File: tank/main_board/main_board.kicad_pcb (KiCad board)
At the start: 2 copper layers, 66.5 x 56.2 mm, 41 parts, among them J1 PowerOut, J10 PowerMotor, J11 SigOut, J12 Spk, J13 LEDs, J14 M0, J15 M1, J16 M2, J2 PowerIn, J3 Encoder0, J4 Encoder1, J5 Encoder2, J6 Encoder3, J7 Bump0, J8 Bump1, J9 Programming Header, U1 L7805, U2 ATMEGA328P-PU, U3 SN74HC595, U4 L293D, U5 L293D, Y1 Crystal

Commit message: debug
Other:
- net class Default removed
- net class Motor removed

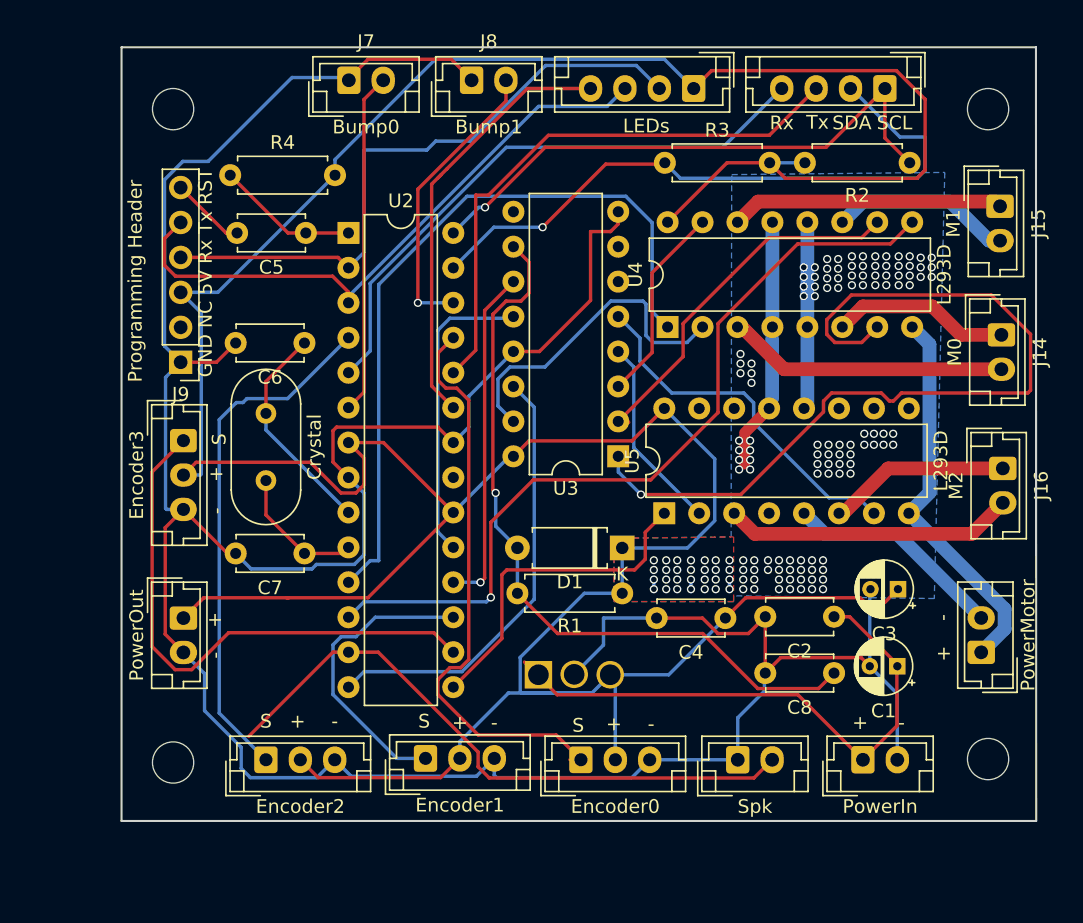
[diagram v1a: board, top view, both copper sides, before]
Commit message: Main Board v0.12
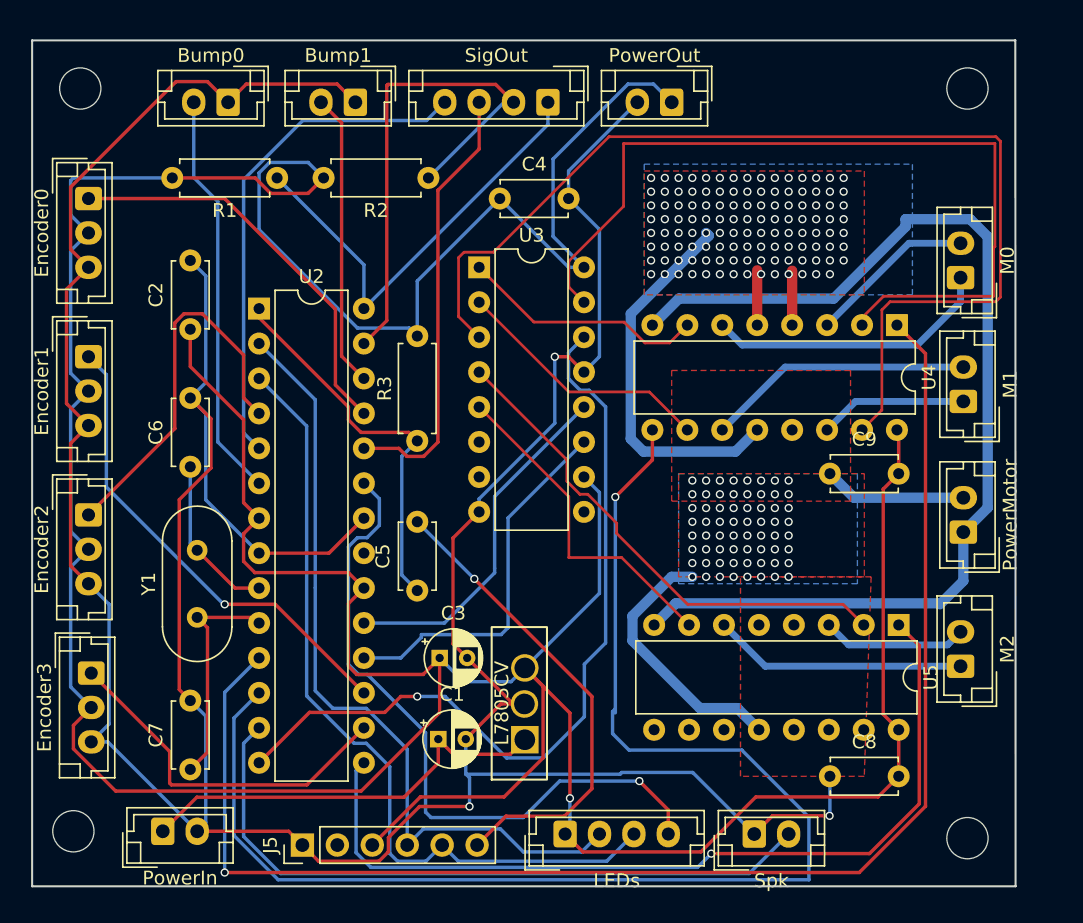
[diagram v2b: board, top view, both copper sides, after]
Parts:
- removed ?: , 
- removed D1: D, custom:D_A-405_P7.62mm_Horizontal
- removed R4: R10, custom:R_Axial_DIN0207_L6.3mm_D2.5mm_P7.62mm_Horizontal
- removed the REF** at (160.5, 125.2)
- removed the REF** at (160.5, 78.0)
- removed the REF** at (101.2, 125.5)
- removed the REF** at (101.2, 78.0)
- added C9: 100nF, custom:C_Disc_D4.7mm_W2.5mm_P5.00mm, F.Cu at (149.0, 104.5)
- added REF**: MountingHole_3mm, custom:MountingHole_3mm, F.Cu at (94.5, 76.5)
- added REF**: MountingHole_3mm, custom:MountingHole_3mm, F.Cu at (159.0, 76.5)
- added REF**: MountingHole_3mm, custom:MountingHole_3mm, F.Cu at (94.0, 130.5)
- added REF**: MountingHole_3mm, custom:MountingHole_3mm, F.Cu at (159.0, 131.0)
- C1: value CP1 -> 10uF
- C2: value C2 -> 100nF
- C3: value CP3 -> 10uF
- C4: value C4 -> 100nF
- C5, C8: value C_Small -> 100nF
- C6: value C6 -> 22pF
- C7: value C7 -> 22pF
- J1: value PowerOut -> Encoder0; footprint custom:JST_EH_B2B-EH-A_1x02_P2.50mm_Vertical -> custom:JST_EH_B3B-EH-A_1x03_P2.50mm_Vertical
- J11: value SigOut -> M0; footprint custom:JST_EH_B4B-EH-A_1x04_P2.50mm_Vertical -> custom:JST_EH_B2B-EH-A_1x02_P2.50mm_Vertical
- J12: value Spk -> M1
- J13: value LEDs -> M2; footprint custom:JST_EH_B4B-EH-A_1x04_P2.50mm_Vertical -> custom:JST_EH_B2B-EH-A_1x02_P2.50mm_Vertical
- J14: value M0 -> Spk
- J15: value M1 -> LEDs; footprint custom:JST_EH_B2B-EH-A_1x02_P2.50mm_Vertical -> custom:JST_EH_B4B-EH-A_1x04_P2.50mm_Vertical
- J16: value M2 -> SigOut; footprint custom:JST_EH_B2B-EH-A_1x02_P2.50mm_Vertical -> custom:JST_EH_B4B-EH-A_1x04_P2.50mm_Vertical
- J2: value PowerIn -> Encoder1; footprint custom:JST_EH_B2B-EH-A_1x02_P2.50mm_Vertical -> custom:JST_EH_B3B-EH-A_1x03_P2.50mm_Vertical
- J3: value Encoder0 -> Encoder2
- J4: value Encoder1 -> Encoder3
- J5: value Encoder2 -> Programming Header; footprint custom:JST_EH_B3B-EH-A_1x03_P2.50mm_Vertical -> custom:PinHeader_1x06_P2.54mm_Vertical
- J6: value Encoder3 -> Bump0; footprint custom:JST_EH_B3B-EH-A_1x03_P2.50mm_Vertical -> custom:JST_EH_B2B-EH-A_1x02_P2.50mm_Vertical
- J7: value Bump0 -> Bump1
- J8: value Bump1 -> PowerOut
- J9: value Programming Header -> PowerIn; footprint custom:PinHeader_1x06_P2.54mm_Vertical -> custom:JST_EH_B2B-EH-A_1x02_P2.50mm_Vertical
- R1: value R -> 10k
- R2: value R7 -> 10k
- R3: value R6 -> 10k
- U1: footprint Custom:L7805CV -> custom:L7805CV
- moved J2 63.5 mm to (95.1, 96.0), turned to -90 degrees
- moved J15 55.5 mm to (129.8, 130.7), turned to 0 degrees
- moved G*** 54.6 mm to (103.6, 81.3)
- moved C2 51.3 mm to (102.5, 94.0), turned to 90 degrees
- moved J13 46.3 mm to (158.5, 118.5), turned to 90 degrees
- moved J16 42.5 mm to (128.5, 77.5), turned to 180 degrees
- moved J14 40.5 mm to (143.5, 130.7), turned to 0 degrees
- moved J3 40.0 mm to (95.1, 107.5), turned to -90 degrees
- moved R1 39.3 mm to (108.8, 83.0)
- moved R2 35.0 mm to (119.8, 83.0)
- moved C4 34.6 mm to (125.0, 84.5), turned to 0 degrees
- moved J9 34.1 mm to (100.5, 130.5), turned to 0 degrees
- moved C1 33.8 mm to (120.5, 123.8), turned to 0 degrees
- moved C3 33.7 mm to (120.6, 117.9), turned to 0 degrees
- moved J1 31.3 mm to (95.1, 84.5)
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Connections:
- C2 pad 1: 9V -> 4.5V
- C8 pad 1: Net-(C8-Pad1) -> GND
- C8 pad 2: GND -> 4.5V
- J1 pad 1: 4.5V -> Encoder0
- J1 pad 2: GND -> 4.5V
- J10 pad 2: Gm -> GND
- J11 pad 1: SCL -> Net-(J11-Pad1)
- J11 pad 2: SDA -> Net-(J11-Pad2)
- J12 pad 1: GND -> Net-(J12-Pad1)
- J12 pad 2: SPK -> Net-(J12-Pad2)
- J13 pad 1: 4.5V -> Net-(J13-Pad1)
- J13 pad 2: LED0 -> Net-(J13-Pad2)
- J14 pad 1: Net-(J14-Pad1) -> GND
- J14 pad 2: Net-(J14-Pad2) -> SPK
- J15 pad 1: Net-(J15-Pad1) -> 4.5V
- J15 pad 2: Net-(J15-Pad2) -> LED0
- J16 pad 1: Net-(J16-Pad1) -> SCL
- J16 pad 2: Net-(J16-Pad2) -> SDA
- J2 pad 1: 9V -> Encoder1
- J2 pad 2: GND -> 4.5V
- J3 pad 1: Encoder0 -> Encoder2
- J4 pad 1: Encoder1 -> Encoder3
- J5 pad 1: Encoder2 -> GND
- J5 pad 2: 4.5V -> unconnected-(J5-Pad2)
- J5 pad 3: GND -> 4.5V
- J6 pad 1: Encoder3 -> GND
- J6 pad 2: 4.5V -> Bump0
- J7 pad 2: Bump0 -> Bump1
- J8 pad 1: GND -> 4.5V
- J8 pad 2: Bump1 -> GND
- J9 pad 1: GND -> 9V
- J9 pad 2: Net-(J9-Pad2) -> GND
- R1 pad 1: 4.5V -> SCL
- R1 pad 2: Net-(C8-Pad1) -> 4.5V
- R2 pad 1: SCL -> SDA
- R3 pad 1: SDA -> Net-(C5-Pad1)
- U2 pad 21: Net-(U2-Pad21) -> unconnected-(U2-Pad21)
- U3 pad 10: Net-(C8-Pad1) -> 4.5V
- U3 pad 6: Net-(U3-Pad6) -> unconnected-(U3-Pad6)
- U3 pad 7: Net-(U3-Pad7) -> unconnected-(U3-Pad7)
- U3 pad 9: Net-(U3-Pad9) -> unconnected-(U3-Pad9)
- U4 pad 11: Net-(J15-Pad2) -> Net-(J12-Pad2)
- U4 pad 12: Gm -> GND
- U4 pad 13: Gm -> GND
- U4 pad 14: Net-(J15-Pad1) -> Net-(J12-Pad1)
- U4 pad 3: Net-(J14-Pad2) -> Net-(J11-Pad2)
- U4 pad 4: Gm -> GND
- U4 pad 5: Gm -> GND
- U4 pad 6: Net-(J14-Pad1) -> Net-(J11-Pad1)
- U5 pad 10: Net-(U5-Pad10) -> unconnected-(U5-Pad10)
- U5 pad 11: Net-(U5-Pad11) -> unconnected-(U5-Pad11)
- U5 pad 12: Gm -> GND
- U5 pad 13: Gm -> GND
- U5 pad 14: Net-(U5-Pad14) -> unconnected-(U5-Pad14)
- U5 pad 15: Net-(U5-Pad15) -> unconnected-(U5-Pad15)
- U5 pad 3: Net-(J16-Pad2) -> Net-(J13-Pad2)
- U5 pad 4: Gm -> GND
- U5 pad 5: Gm -> GND
- U5 pad 6: Net-(J16-Pad1) -> Net-(J13-Pad1)
- U5 pad 9: Net-(U5-Pad9) -> unconnected-(U5-Pad9)
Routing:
- net GND: track 228.1 -> 334.4 mm, vias 0 -> 186
- net M1-: track 14.5 -> 79.2 mm
- net Net-(C8-Pad1): track 54.5 -> 0.00 mm, vias 1 -> 0
- net M0PWM: track 54.3 -> 105.4 mm, vias 0 -> 1
- net Vm: track 28.4 -> 77.9 mm
- net Gm: track 48.4 -> 0.00 mm, vias 142 -> 0
- net 4.5V: track 272.2 -> 319.9 mm, vias 0 -> 1
- net M0-: track 62.1 -> 18.0 mm, vias 1 -> 0
- net M1PWM: track 59.9 -> 99.2 mm
- net M2PWM: track 24.4 -> 63.7 mm, vias 0 -> 1
- net M0+: track 24.2 -> 62.5 mm
- net Net-(C5-Pad2): track 5.47 -> 34.7 mm, vias 0 -> 1
- net SERIAL_DATA: track 32.3 -> 58.9 mm, vias 0 -> 1
- net M2+: track 14.2 -> 36.9 mm
- net Net-(J16-Pad2): track 21.1 -> 0.00 mm
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- added copper zone on B.Cu, net GND
- added copper zone on F.Cu, net GND
- removed copper zone on B.Cu, net Gm
- removed copper zone on F.Cu, net Gm
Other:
- board size 66.5 x 56.2 mm -> 71.5 x 61.5 mm
- board text added: "Main Board v0.12 Laser Tag Robot Tank M.I.A.R. Labs nick.groesz@gmail.com"
- board text removed: "+"
- board text removed: "-"
- board text removed: "GND NC 5V Rx Tx RST"
- board text removed: "Laser Tag Robot Tank Main Board v0.11 M.I.A.R. Labs nick.groesz@gmail.com"
- board text removed: "Rx"
- board text removed: "S"
- board text removed: "SCL"
- board text removed: "SDA"
- board text removed: "Tx"
